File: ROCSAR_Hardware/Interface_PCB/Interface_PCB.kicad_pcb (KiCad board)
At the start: 2 copper layers, 240 x 100 mm, 35 parts, among them J1 Remove Before Flight, J2 USB_A, J3 USB_A, U1 TEN 60-2422N, U2 LM2576-5.0WU, U3 LM2576-5.0WU, U4 LM2576-5.0WU, U5 LM2576-5.0WU

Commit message: Interface PCB mostly done
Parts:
- removed J3: USB_A, Connector_USB:USB_A_Molex_67643_Horizontal
- added A1: RaspberryPi_Pico, Module:RaspberryPi_Pico_Common_Unspecified, F.Cu at (189.8, 109.4)
- added C1: 100uF, Capacitor_SMD:C_1206_3216Metric_Pad1.33x1.80mm_HandSolder, F.Cu at (170.6, 57.9)
- added C13: C_Small, Capacitor_SMD:C_0603_1608Metric_Pad1.08x0.95mm_HandSolder, F.Cu at (169.9, 129.8)
- added C14: C_Small, Capacitor_SMD:C_0603_1608Metric_Pad1.08x0.95mm_HandSolder, F.Cu at (162.6, 100.6)
- added C15: 1uF, Capacitor_SMD:C_0603_1608Metric_Pad1.08x0.95mm_HandSolder, F.Cu at (196.8, 71.7)
- added C16: 100nF, Capacitor_SMD:C_0603_1608Metric_Pad1.08x0.95mm_HandSolder, F.Cu at (200.7, 80.0)
- added C17: 120nF, Capacitor_SMD:C_0603_1608Metric_Pad1.08x0.95mm_HandSolder, F.Cu at (197.8, 80.0)
- added C2: 330uF, Capacitor_SMD:C_1206_3216Metric_Pad1.33x1.80mm_HandSolder, F.Cu at (180.4, 77.8)
- added D6: 1N5822, 1N5822:DIOAD2120W130L950D530P, F.Cu at (169.9, 71.3)
- added IC1: SN74LVC1G123DCTT, SN74LVC1G123DCTT:SOP65P400X130-8N, F.Cu at (168.2, 123.4)
- added IC2: SN74LVC1G123DCTT, SN74LVC1G123DCTT:SOP65P400X130-8N, F.Cu at (164.1, 106.9)
- added J4: RJE05188051C, RJE05188051C:RJE05188051C, F.Cu at (70.6, 120.1)
- added J5: RJE05188051C, RJE05188051C:RJE05188051C, B.Cu at (70.5, 51.4)
- added J6: USB1086-GF-B, USB1086-GF-B:USB1086GFB, B.Cu at (210.6, 40.4)
- added J7: USB1086-GF-B, USB1086-GF-B:USB1086GFB, F.Cu at (210.5, 131.0)
- added JP1: Jumper_2_Open, Jumper:SolderJumper-2_P1.3mm_Open_RoundedPad1.0x1.5mm, F.Cu at (201.3, 73.2)
- added L5: 330uH, SRR1050HA-331Y:INDPM102100X510N, F.Cu at (178.8, 70.4)
- added Q1: PBSS5250PAS-QX, PBSS5250PAS-QX:PMEG2020EPASX, F.Cu at (165.2, 129.4)
- added Q2: PBSS5250PAS-QX, PBSS5250PAS-QX:PMEG2020EPASX, F.Cu at (185.7, 54.4)
- added Q3: PBSS5250PAS-QX, PBSS5250PAS-QX:PMEG2020EPASX, F.Cu at (167.1, 101.0)
- added R10: 100K, Resistor_SMD:R_0603_1608Metric_Pad0.98x0.95mm_HandSolder, F.Cu at (189.5, 55.8)
- added R11: 10K, Resistor_SMD:R_0603_1608Metric_Pad0.98x0.95mm_HandSolder, F.Cu at (189.5, 52.8)
- added R12: 22K, Resistor_SMD:R_0603_1608Metric_Pad0.98x0.95mm_HandSolder, F.Cu at (190.4, 50.3)
- added R13: 2K2, Resistor_SMD:R_0603_1608Metric_Pad0.98x0.95mm_HandSolder, F.Cu at (183.9, 43.8)
- added R14: 5K6, Resistor_SMD:R_0603_1608Metric_Pad0.98x0.95mm_HandSolder, F.Cu at (184.5, 58.2)
- added R15: 2K2, Resistor_SMD:R_0603_1608Metric_Pad0.98x0.95mm_HandSolder, F.Cu at (187.3, 58.2)
- added R16: 2K2, Resistor_SMD:R_0603_1608Metric_Pad0.98x0.95mm_HandSolder, F.Cu at (186.4, 60.8)
- added R17: 5K6, Resistor_SMD:R_0603_1608Metric_Pad0.98x0.95mm_HandSolder, F.Cu at (191.2, 46.0)
- added R18: 10K, Resistor_SMD:R_0603_1608Metric_Pad0.98x0.95mm_HandSolder, F.Cu at (193.7, 45.1)
- added R19: NI, Resistor_SMD:R_0603_1608Metric_Pad0.98x0.95mm_HandSolder, F.Cu at (187.3, 43.8)
- added R20: NI, Resistor_SMD:R_0603_1608Metric_Pad0.98x0.95mm_HandSolder, F.Cu at (183.9, 40.9)
- added R21: 2K2, Resistor_SMD:R_0603_1608Metric_Pad0.98x0.95mm_HandSolder, F.Cu at (191.2, 47.7)
- added R22: 3.09K, Resistor_SMD:R_1206_3216Metric_Pad1.30x1.75mm_HandSolder, F.Cu at (174.6, 61.8)
- added R23: 1K, Resistor_SMD:R_1206_3216Metric_Pad1.30x1.75mm_HandSolder, F.Cu at (175.9, 57.9)
- added R24: R_Small, Resistor_SMD:R_0603_1608Metric_Pad0.98x0.95mm_HandSolder, F.Cu at (169.8, 127.0)
- added R25: 100K, Resistor_SMD:R_0603_1608Metric_Pad0.98x0.95mm_HandSolder, F.Cu at (164.2, 122.5)
- added R26: 10K, Resistor_SMD:R_0603_1608Metric_Pad0.98x0.95mm_HandSolder, F.Cu at (164.2, 125.3)
- added R27: 4K7, Resistor_SMD:R_0603_1608Metric_Pad0.98x0.95mm_HandSolder, F.Cu at (166.6, 133.2)
- added R28: 3K3, Resistor_SMD:R_0603_1608Metric_Pad0.98x0.95mm_HandSolder, F.Cu at (163.7, 133.2)
- added R29: ~, Resistor_SMD:R_0603_1608Metric_Pad0.98x0.95mm_HandSolder, F.Cu at (168.2, 119.2)
- added R30: R_Small, Resistor_SMD:R_0603_1608Metric_Pad0.98x0.95mm_HandSolder, F.Cu at (168.2, 116.2)
- added R31: R_Small, Resistor_SMD:R_0603_1608Metric_Pad0.98x0.95mm_HandSolder, F.Cu at (168.2, 113.2)
- added R32: R_Small, Resistor_SMD:R_0603_1608Metric_Pad0.98x0.95mm_HandSolder, F.Cu at (164.1, 117.2)
- added R33: R_Small, Resistor_SMD:R_0603_1608Metric_Pad0.98x0.95mm_HandSolder, F.Cu at (164.0, 114.2)
- added R34: ~, Resistor_SMD:R_0603_1608Metric_Pad0.98x0.95mm_HandSolder, F.Cu at (164.1, 111.2)
- added R35: 100K, Resistor_SMD:R_0603_1608Metric_Pad0.98x0.95mm_HandSolder, F.Cu at (167.7, 107.8)
- added R36: R_Small, Resistor_SMD:R_0603_1608Metric_Pad0.98x0.95mm_HandSolder, F.Cu at (162.5, 103.3)
- added R37: 10K, Resistor_SMD:R_0603_1608Metric_Pad0.98x0.95mm_HandSolder, F.Cu at (167.7, 105.0)
- added R38: 3K3, Resistor_SMD:R_0603_1608Metric_Pad0.98x0.95mm_HandSolder, F.Cu at (168.6, 97.2)
- added R39: 4K7, Resistor_SMD:R_0603_1608Metric_Pad0.98x0.95mm_HandSolder, F.Cu at (165.6, 97.2)
- added R40: 10K, Resistor_SMD:R_0603_1608Metric_Pad0.98x0.95mm_HandSolder, F.Cu at (200.7, 76.6)
- added R41: 10K, Resistor_SMD:R_0603_1608Metric_Pad0.98x0.95mm_HandSolder, F.Cu at (193.7, 71.7)
- added R42: TBD, Resistor_SMD:R_0603_1608Metric_Pad0.98x0.95mm_HandSolder, F.Cu at (192.2, 78.7)
- added R43: TBD, Resistor_SMD:R_0603_1608Metric_Pad0.98x0.95mm_HandSolder, F.Cu at (191.3, 76.3)
- added R9: 10K, Resistor_SMD:R_0603_1608Metric_Pad0.98x0.95mm_HandSolder, F.Cu at (193.0, 49.3)
- added U6: SN74HC126PWR, KiCADv6:PW14, F.Cu at (185.4, 47.4)
- added U7: LM2576-5.0WU, LM2576-5.0WU:MICROCHIP_TO-263, F.Cu at (172.6, 40.2)
- added U8: BNO055, BNO055:LGA28R50P4X10_380X520X100, F.Cu at (196.0, 76.0)
- D5: value 1N5822 -> V10P6HM3_A_H; footprint 1N5822:DIOAD2120W130L950D530P -> V10P6HM3_A_H:V10P6HM3_AH; moved to B.Cu
- J1: value Remove Before Flight -> 1803277; footprint Connector_PinHeader_2.54mm:PinHeader_1x02_P2.54mm_Vertical -> 1803277:PHOENIX_1803277; moved to F.Cu
- J2: value USB_A -> 1757242; footprint Connector_USB:USB_A_Molex_67643_Horizontal -> 1757242:PHOENIX_1757242
- moved J2 193.4 mm to (99.5, 135.1), turned to 0 degrees
- moved J1 54.7 mm to (84.3, 135.1), turned to 0 degrees
- moved C8 44.2 mm to (158.6, 127.9)
- moved U5 43.8 mm to (128.2, 40.2)
- moved C6 43.7 mm to (158.4, 77.8)
- moved D2 43.7 mm to (147.8, 71.3)
- moved L4 43.7 mm to (134.8, 70.6)
- moved R6 43.7 mm to (132.8, 108.4)
- moved R8 43.7 mm to (131.8, 58.1)
- moved C4 43.7 mm to (106.5, 44.9)
- moved U1 43.7 mm to (105.5, 98.4)
- moved C10 43.7 mm to (137.3, 128.1)
- moved C11 43.7 mm to (126.5, 58.1)
- moved C12 43.7 mm to (136.2, 78.0)
- moved C3 43.7 mm to (106.5, 48.6)
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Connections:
- net Net-(C10-Pad2) renamed +5V RX
- net Net-(C12-Pad2) renamed +5V TX
- net Net-(C6-Pad2) renamed +5V GNSS
- net Net-(C8-Pad2) renamed +5V Servo
- U1 pad 1: Net-(U1-+VIN(VCC)) -> Net-(D5-K)
- U1 pad 3: Net-(J1-Pin_1) -> Net-(U1-REMOTE_ON/OFF)
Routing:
- net +5V Main: track 0.00 -> 129.3 mm, vias 0 -> 3
- net +12V: track 149.0 -> 252.4 mm, vias 4 -> 7
- net Net-(J6-MH1): track 0.00 -> 92.0 mm
- net Net-(J6-MH2): track 0.00 -> 91.9 mm
- net Net-(J6-GND): track 0.00 -> 91.1 mm
- net Net-(J6-VBUS): track 0.00 -> 91.0 mm
- net Net-(J6-D-): track 0.00 -> 90.6 mm
- net Net-(J6-D+): track 0.00 -> 90.6 mm
- net Net-(J2-D-): track 90.2 -> 0.00 mm
- net Net-(J6-STDA_SSTX+): track 0.00 -> 87.8 mm
- net Net-(J6-STDA_SSTX-): track 0.00 -> 87.6 mm
- net Net-(J6-STDA_SSRX-): track 0.00 -> 87.6 mm
- net Net-(J6-STDA_SSRX+): track 0.00 -> 87.6 mm
- net Net-(J6-GND_DRAIN): track 0.00 -> 87.6 mm
- net Net-(J2-VBUS): track 84.2 -> 0.00 mm
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- removed copper zone on B.Cu, net -VDC
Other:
- board size 240 x 100 mm -> 160 x 100 mm
- board text added: "- | +"

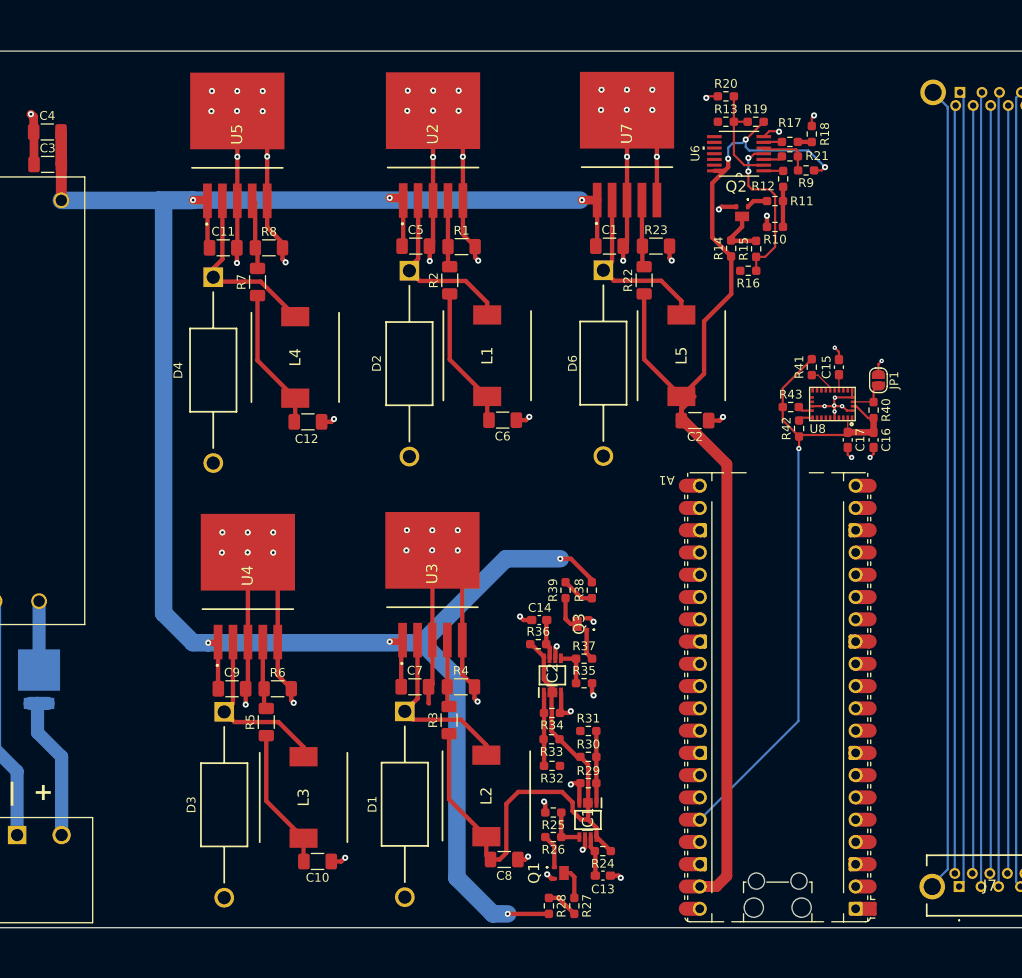
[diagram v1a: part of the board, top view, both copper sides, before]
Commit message: atualizacoes interface
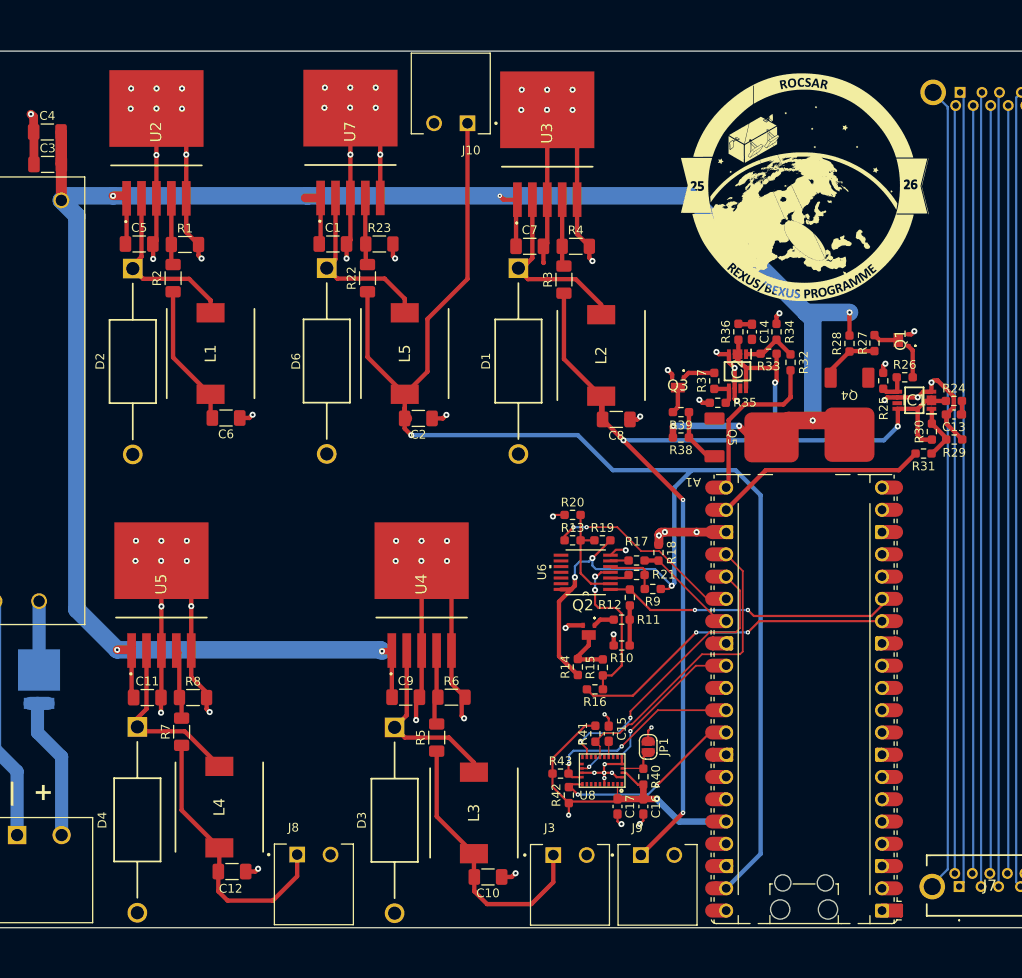
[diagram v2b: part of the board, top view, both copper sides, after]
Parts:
- added G***: LOGO, ROCSAR_Logo:aaa, F.Cu at (179.1, 83.1)
- added J10: 1803277, 1803277:PHOENIX_1803277, F.Cu at (157.0, 35.9)
- added J3: 1803277, 1803277:PHOENIX_1803277, F.Cu at (161.6, 135.4)
- added J8: 1803277, 1803277:PHOENIX_1803277, F.Cu at (132.4, 135.3)
- added J9: 1803277, 1803277:PHOENIX_1803277, F.Cu at (171.6, 135.4)
- added Q4: SIHFR9024, SIHFR9024:SIHFR9024, F.Cu at (198.0, 74.5)
- added Q5: SIHFR9024, SIHFR9024:SIHFR9024, F.Cu at (184.1, 79.8)
- moved R27 72.8 mm to (200.8, 69.0)
- moved R28 72.7 mm to (198.0, 69.0), turned to 90 degrees
- moved Q1 72.0 mm to (203.7, 68.7), turned to 90 degrees
- moved C13 66.1 mm to (209.9, 77.1), turned to 180 degrees
- moved R26 66.0 mm to (204.3, 72.9), turned to 0 degrees
- moved R24 65.1 mm to (209.9, 75.6), turned to 0 degrees
- moved R25 62.0 mm to (201.8, 73.3), turned to 90 degrees
- moved IC1 60.7 mm to (205.4, 75.5), turned to 180 degrees
- moved R29 57.3 mm to (209.9, 80.0), turned to 0 degrees
- moved R30 54.0 mm to (207.4, 79.1), turned to 90 degrees
- moved R32 53.5 mm to (191.3, 71.2), turned to 90 degrees
- moved D1 52.2 mm to (160.2, 71.1)
- moved L4 52.0 mm to (126.1, 121.9)
- moved C11 52.0 mm to (117.9, 109.4)
- moved R8 52.0 mm to (123.1, 109.4)
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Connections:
- A1 pad 14: unconnected-(A1-GPIO10-Pad14) -> RX_EN
- A1 pad 15: unconnected-(A1-GPIO11-Pad15) -> TX_EN
- A1 pad 21: unconnected-(A1-GPIO16-Pad21) -> MCU_HEAT_2
- A1 pad 22: unconnected-(A1-GPIO17-Pad22) -> MCU_HEAT_1
- A1 pad 24: unconnected-(A1-GPIO18-Pad24) -> N_RESET
- A1 pad 25: unconnected-(A1-GPIO19-Pad25) -> INT
- A1 pad 26: unconnected-(A1-GPIO20-Pad26) -> UART TX
- A1 pad 27: unconnected-(A1-GPIO21-Pad27) -> UART RX
- A1 pad 29: unconnected-(A1-GPIO22-Pad29) -> I2C_ADDR_SEL
- A1 pad 31: unconnected-(A1-GPIO26_ADC0-Pad31) -> SDA
- A1 pad 32: unconnected-(A1-GPIO27_ADC1-Pad32) -> SCL
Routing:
- net +5V Servo: track 64.9 -> 140.0 mm, vias 0 -> 5
- net +5V Main: track 129.3 -> 189.9 mm, vias 3 -> 4
- net RX_EN: track 0.00 -> 37.5 mm, vias 0 -> 2
- net +3.3V: track 74.3 -> 39.2 mm, vias 1 -> 2
- net INT: track 0.00 -> 32.7 mm, vias 0 -> 2
- net N_RESET: track 3.02 -> 34.9 mm
- net TX_EN: track 2.22 -> 33.5 mm, vias 0 -> 2
- net MCU_HEAT_1: track 0.00 -> 24.3 mm
- net UART TX: track 0.00 -> 22.7 mm, vias 0 -> 2
- net I2C_ADDR_SEL: track 0.00 -> 22.3 mm, vias 0 -> 2
- net SDA: track 1.69 -> 23.9 mm, vias 0 -> 2
- net SCL: track 1.68 -> 22.9 mm, vias 0 -> 2
- net MCU_HEAT_2: track 0.00 -> 19.0 mm
- net GND: track 233.7 -> 252.7 mm, vias 75 -> 78
- net +5V RX: track 16.1 -> 31.5 mm
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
